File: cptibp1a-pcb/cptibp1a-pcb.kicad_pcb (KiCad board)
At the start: 2 copper layers, 50.5 x 42 mm, 29 parts, among them J1 10118194-0001LF, J2 PAD+, J3 PAD-, Q1 2N7002, Q2 AO3413, U1 NCP360SNT, U2 APX809S-31SA, U3 BQ21040, U4 APX810S-44SA, U5 NCP380HSN05

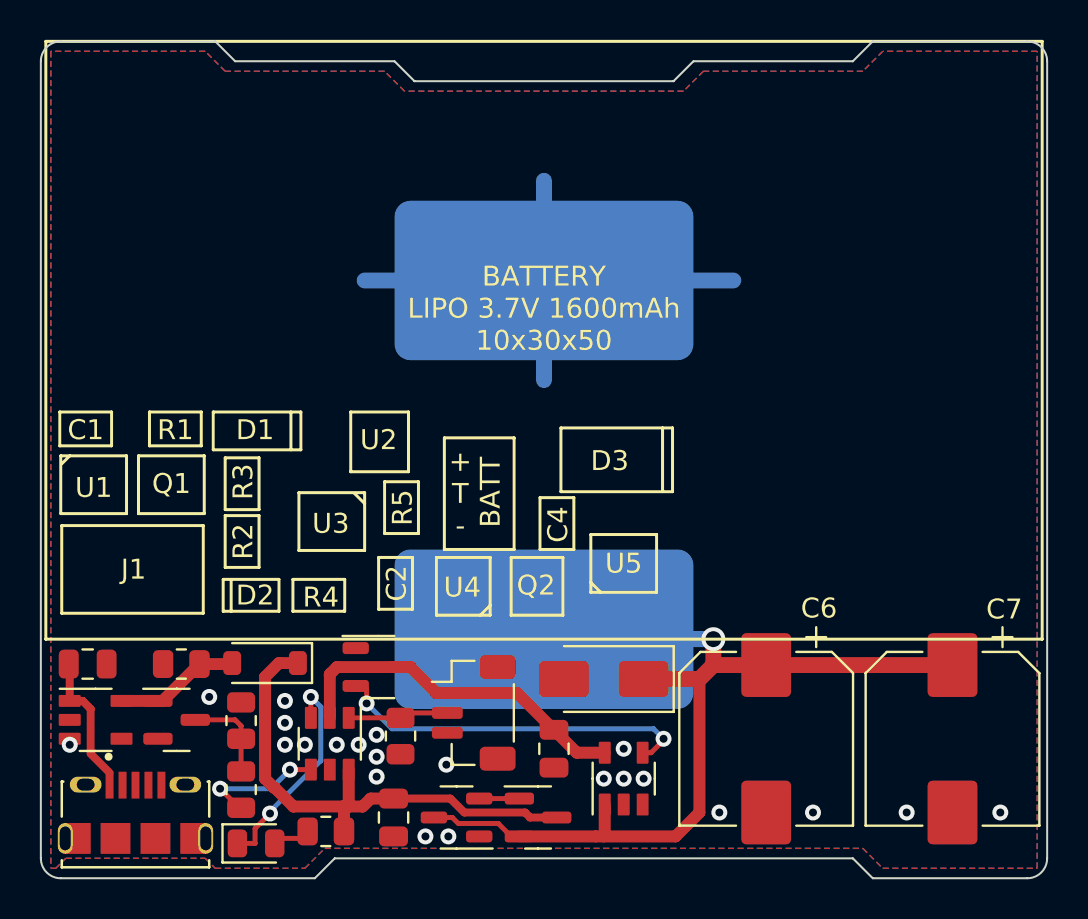
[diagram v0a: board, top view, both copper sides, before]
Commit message: rev1
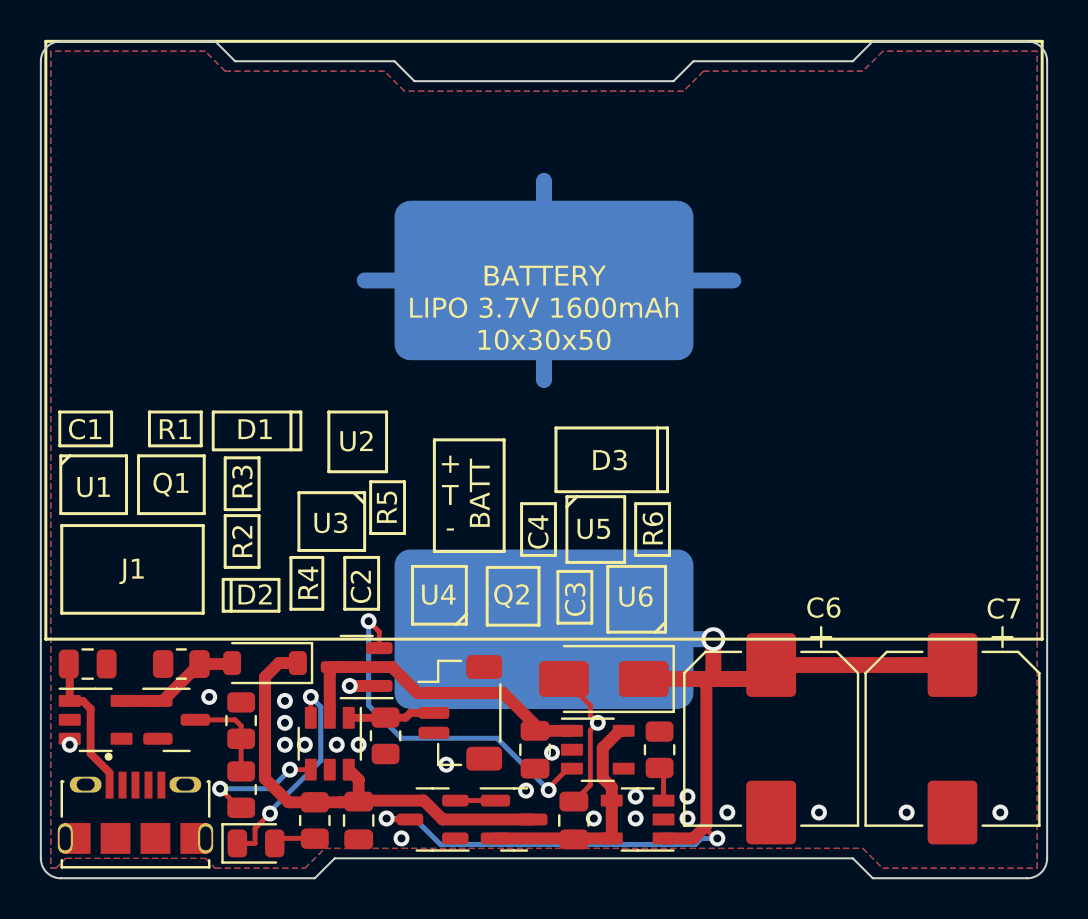
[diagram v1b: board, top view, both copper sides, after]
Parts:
- added C3: 4u7, Capacitor_SMD:C_0805_2012Metric, F.Cu at (1.50, 39.1)
- added R6: 10k, Resistor_SMD:R_0805_2012Metric, F.Cu at (5.80, 35.5)
- added U6: NCP380HSN05, george:SOT-23-5_TI_DBV5, F.Cu at (4.70, 39.0)
- U5: value NCP380HSN05 -> MAX40203AUK
- moved U5 1.95 mm to (2.70, 35.5), turned to 0 degrees
- moved C2 1.76 mm to (-9.30, 39.1)
- moved U4 1.20 mm to (-5.59, 39.0)
- moved Q2 1.20 mm to (-1.50, 39.0)
- moved U2 1.09 mm to (-9.40, 31.4), turned to 180 degrees
- moved C4 0.95 mm to (-0.45, 35.5)
- moved R4 0.78 mm to (-11.5, 39.1), turned to 90 degrees
- moved R5 0.75 mm to (-7.95, 34.9)
- moved BT1 0.68 mm to (-4.20, 33.7)
- moved C6 0.25 mm to (11.4, 35.0)
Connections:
- C6 pad 1: /VOUT -> /VOUTF
- C7 pad 1: /VOUT -> /VOUTF
- D3 pad 1: /VOUT -> /VOUTF
- J2 pad 1: /VOUT -> /VOUTF
- U4 pad 3: /VOUT -> /VOUTF
- U5 pad 1: /VOUT -> /B+
- U5 pad 3: unconnected-(U5-~{OC}-Pad3) -> /EN
- U5 pad 4: /EN -> unconnected-(U5-NC-Pad4)
- U5 pad 5: /B+ -> /VOUT
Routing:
- net /VOUTF: track 0.00 -> 55.6 mm, vias 0 -> 3
- net /VOUT: track 47.7 -> 12.0 mm, vias 1 -> 0
- net /GND: track 28.5 -> 37.3 mm, vias 22 -> 23
- net /VCC: track 25.9 -> 23.4 mm
- net Net-(U6-~{OC}): track 0.00 -> 1.72 mm
- net /B+: track 17.4 -> 16.2 mm
